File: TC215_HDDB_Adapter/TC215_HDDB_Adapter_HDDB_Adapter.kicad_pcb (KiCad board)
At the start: 2 copper layers, 19 x 66.7 mm, 4 parts, among them J1 Conn_02x25_Odd_Even, J2 DB25_Female

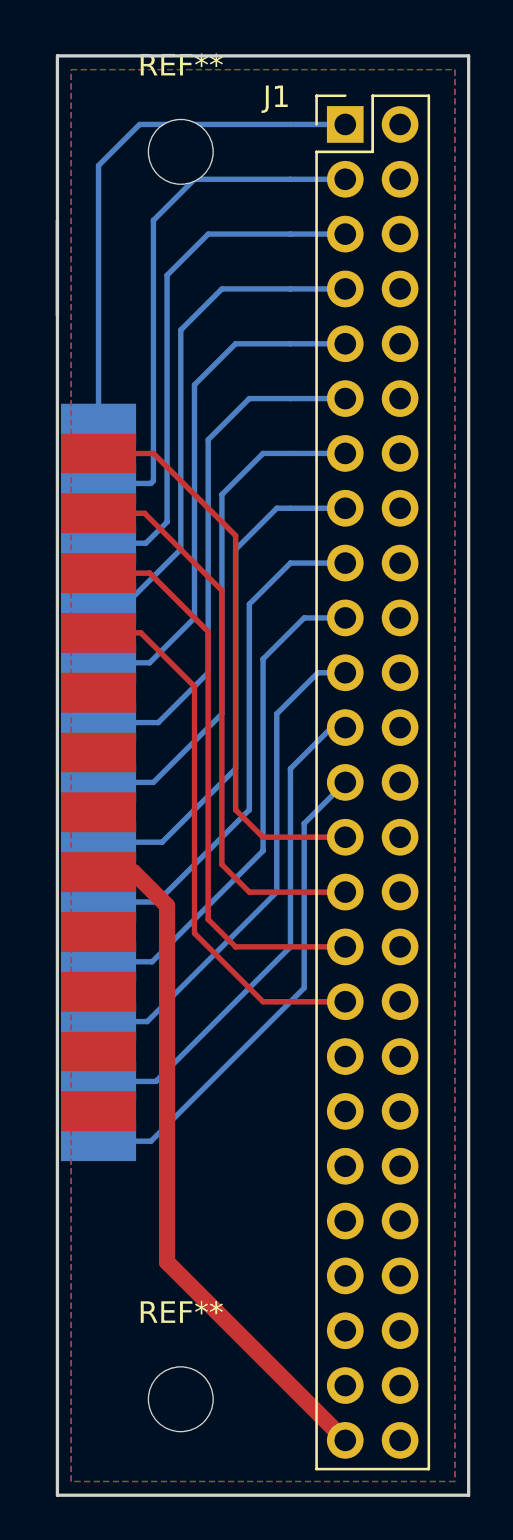
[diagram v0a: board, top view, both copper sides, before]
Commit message: adapter design ready
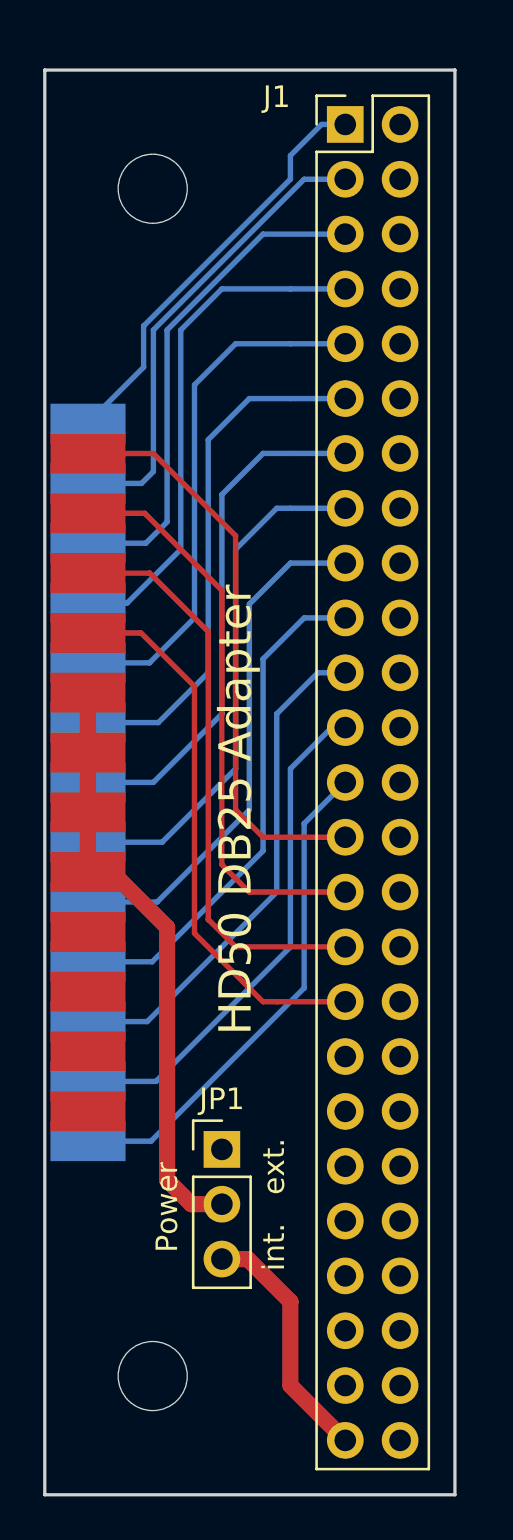
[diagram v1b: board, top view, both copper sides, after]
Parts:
- removed the REF** at (81.3, 83.8)
- removed the REF** at (81.3, 141.6)
- added JP1: Jumper_NC_Dual, Pin_Headers:Pin_Header_Straight_1x03_Pitch2.54mm, F.Cu at (83.2, 130.0)
- added REF**: MountingHole_3.2mm_M3_ISO7380, Mounting_Holes:MountingHole_3.2mm_M3_ISO7380, F.Cu at (80.0, 85.5)
- added REF**: MountingHole_3.2mm_M3_ISO7380, Mounting_Holes:MountingHole_3.2mm_M3_ISO7380, F.Cu at (80.0, 140.5)
- moved J2 0.49 mm to (77.0, 113.0)
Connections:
- J2 pad 18: Net-(J1-Pad49) -> Net-(J2-Pad18)
- J2 pad 19: Net-(J1-Pad49) -> Net-(J2-Pad18)
- J2 pad 20: Net-(J1-Pad49) -> Net-(J2-Pad18)
- J2 pad 21: Net-(J1-Pad49) -> Net-(J2-Pad18)
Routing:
- net Net-(J2-Pad18): track 0.00 -> 27.7 mm
- net Net-(J1-Pad49): track 32.0 -> 11.5 mm
- net Net-(J1-Pad1): track 24.2 -> 19.2 mm
- net Net-(J1-Pad3): track 23.7 -> 21.1 mm
- net Net-(J1-Pad5): track 23.4 -> 21.9 mm
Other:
- board size 19 x 66.7 mm -> 19 x 66 mm
- board text added: "HD50 DB25 Adapter"
- board text added: "Power"
- board text added: "int. ext."
